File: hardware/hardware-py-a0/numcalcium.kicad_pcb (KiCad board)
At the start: 2 copper layers, 77.6 x 158.1 mm, 111 parts, among them J1 Conn_02x08_Odd_Even, J12 Micro_SD_Card_Det2, J2 USB_C_Receptacle_USB2.0_16P, J3 Conn_02x04_Odd_Even, J4 LCD_socket, J9 AudioJack4, Q1 AO3401A, Q2 AO3401A, Q3 AO3401A, Q6 BSS138, Q7 AO3401A, Q8 BSS138, Q9 BSS138, SW1 SW_Push, SW10 SW_Push, SW11 SW_Push, SW12 SW_Push, SW13 SW_Push, SW14 SW_Push, SW15 SW_Push, SW16 SW_Push, SW17 SW_Push, SW18 SW_Push, SW19 SW_Push, SW2 SW_Push, SW20 SW_Push, SW21 Encoder, SW22 RST, SW3 SW_Push, SW4 SW_Push, SW5 SW_Push, SW6 SW_Push, SW7 SW_Push, SW8 SW_Push, SW9 SW_Push, U1 LTC4054ES5-4.2, U2 STI3411A, U3 74HC595, U4 ESP32-S3-WROOM-1, U6 XC6206PxxxMR

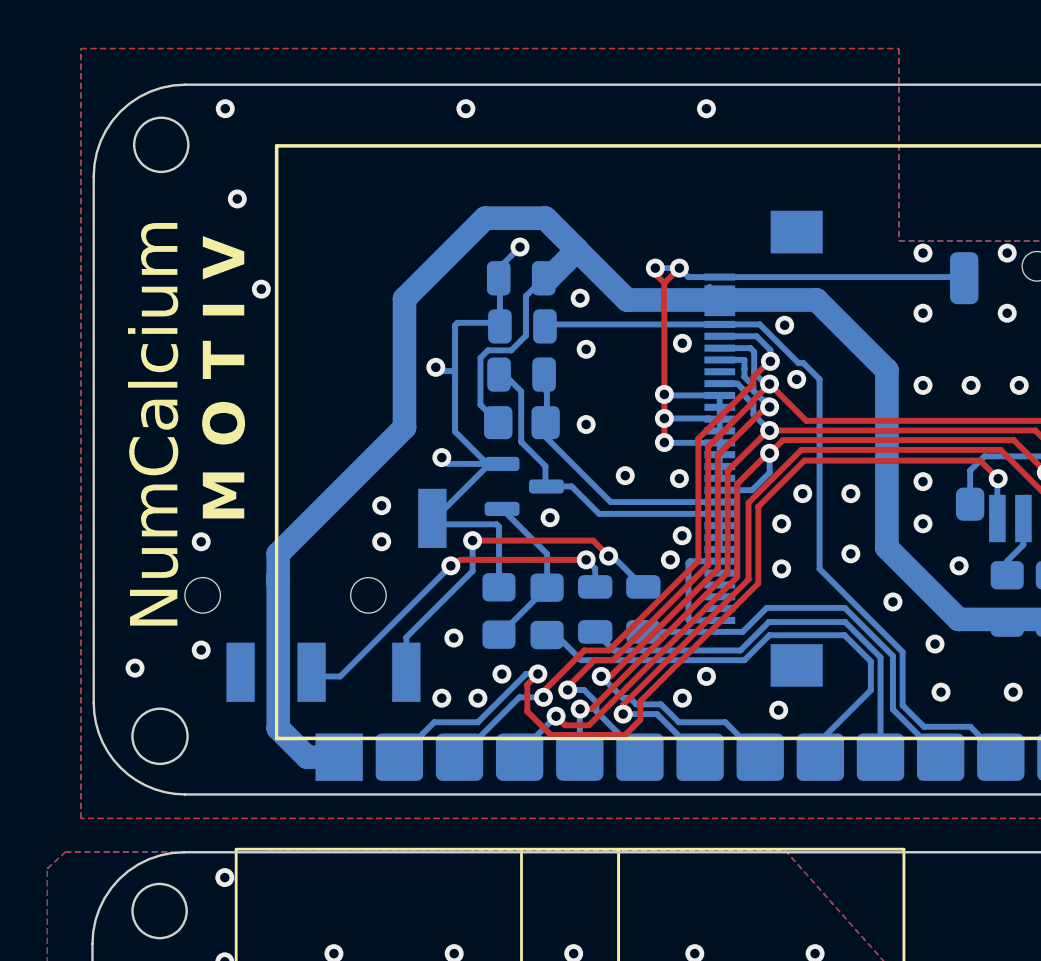
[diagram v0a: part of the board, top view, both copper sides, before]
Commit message: [dev] py-a0 board files
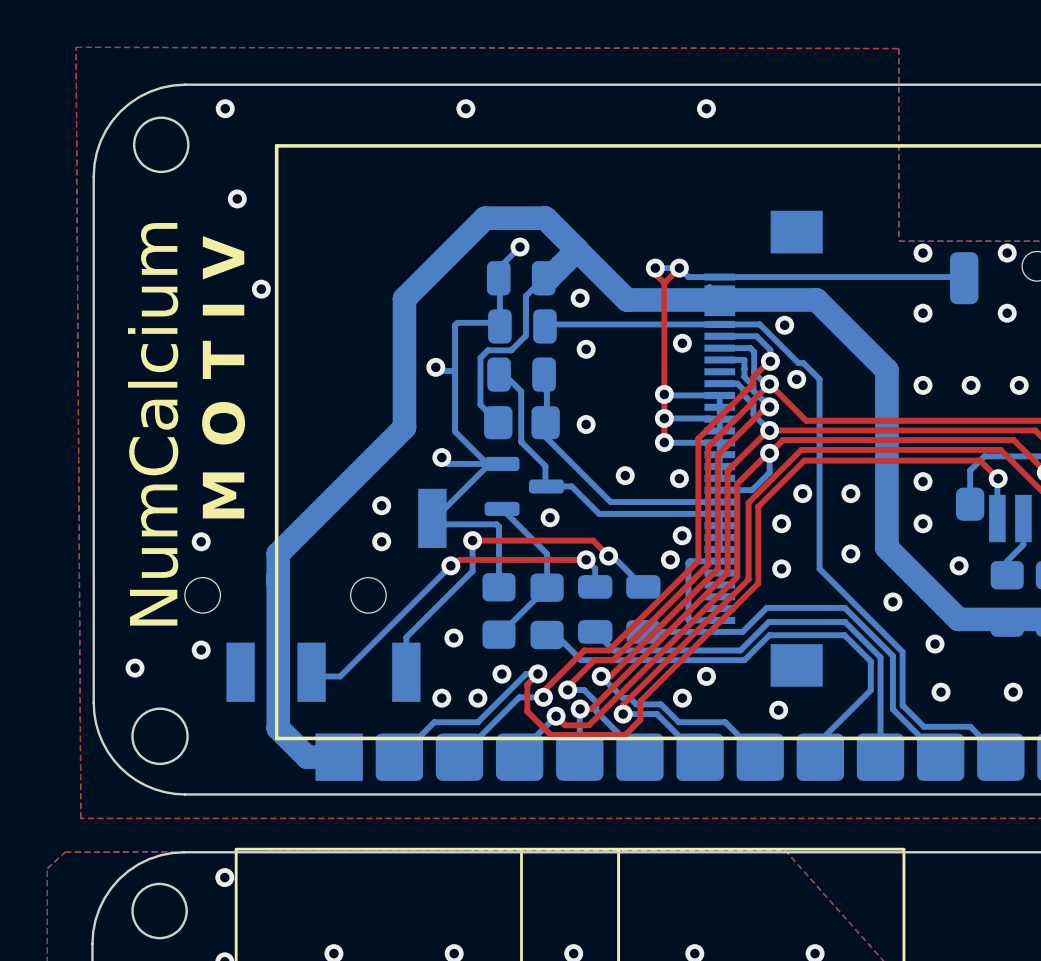
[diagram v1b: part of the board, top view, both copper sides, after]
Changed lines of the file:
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@@
 		(tags "SOT TO_SOT_SMD")
 		(property "Reference" "U6"
-			(at -0.508 0 360)
+			(at -0.508 0 0)
 			(layer "F.SilkS")
 			(effects
@@
 		)
 		(property "Value" "XC6206PxxxMR"
-			(at 0 2.4 360)
+			(at 0 2.4 0)
 			(layer "F.Fab")
 			(effects
@@
 		)
 		(fp_text user "${REFERENCE}"
-			(at 0 0 360)
+			(at 0 0 0)
 			(layer "F.Fab")
 			(effects
@@
 		(tags "diode handsolder")
 		(property "Reference" "D24"
-			(at -0.009 0.0254 360)
+			(at -0.009 0.0254 0)
 			(layer "F.SilkS")
 			(effects
@@
 		(tags "SOT TO_SOT_SMD")
 		(property "Reference" "Q3"
-			(at -0.6835 0 360)
+			(at -0.6835 0 0)
 			(layer "F.SilkS")
 			(effects
@@
 		)
 		(property "Value" "AO3401A"
-			(at 0 2.4 360)
+			(at 0 2.4 0)
 			(layer "F.Fab")
 			(effects
@@
 		)
 		(fp_text user "${REFERENCE}"
-			(at 0 0 360)
+			(at 0 0 0)
 			(layer "F.Fab")
 			(effects
@@
 		)
 		(fp_text user "+"
-			(at -1.326 4.9836 360)
+			(at -1.326 4.9836 0)
 			(layer "B.SilkS")
 			(effects
@@
 		)
 		(fp_text user "+"
-			(at -2.75 2.75 360)
+			(at -2.75 2.75 0)
 			(layer "B.Fab")
 			(effects
@@
 		(tags "diode handsolder")
 		(property "Reference" "D27"
-			(at 0 -0.0254 360)
+			(at 0 -0.0254 0)
 			(layer "B.SilkS")
 			(effects
@@
 		(polygon
 			(pts
-				(xy -1.016 -35.56) (xy 33.528 -35.56) (xy 33.528 -27.432) (xy 57.912 -27.432) (xy 57.912 -3.048)
+				(xy -1.2192 -35.6108) (xy 33.528 -35.56) (xy 33.528 -27.432) (xy 57.912 -27.432) (xy 57.912 -3.048)
 				(xy -1.016 -3.048)
 			)
